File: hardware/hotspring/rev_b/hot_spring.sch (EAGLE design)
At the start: 27 parts, among them J1 GECKO_POWER_SUPPLY_CONN, J2 JUMPER-31-2, Q1 MOSFET-NCHANNELSMD, Q2 MOSFET-NCHANNELSMD, Q3 DUAL_MOSFET_NP, T1 LPR6235-752SMR, T2 LPR6235-752SMR, U1 LTC3109EUF

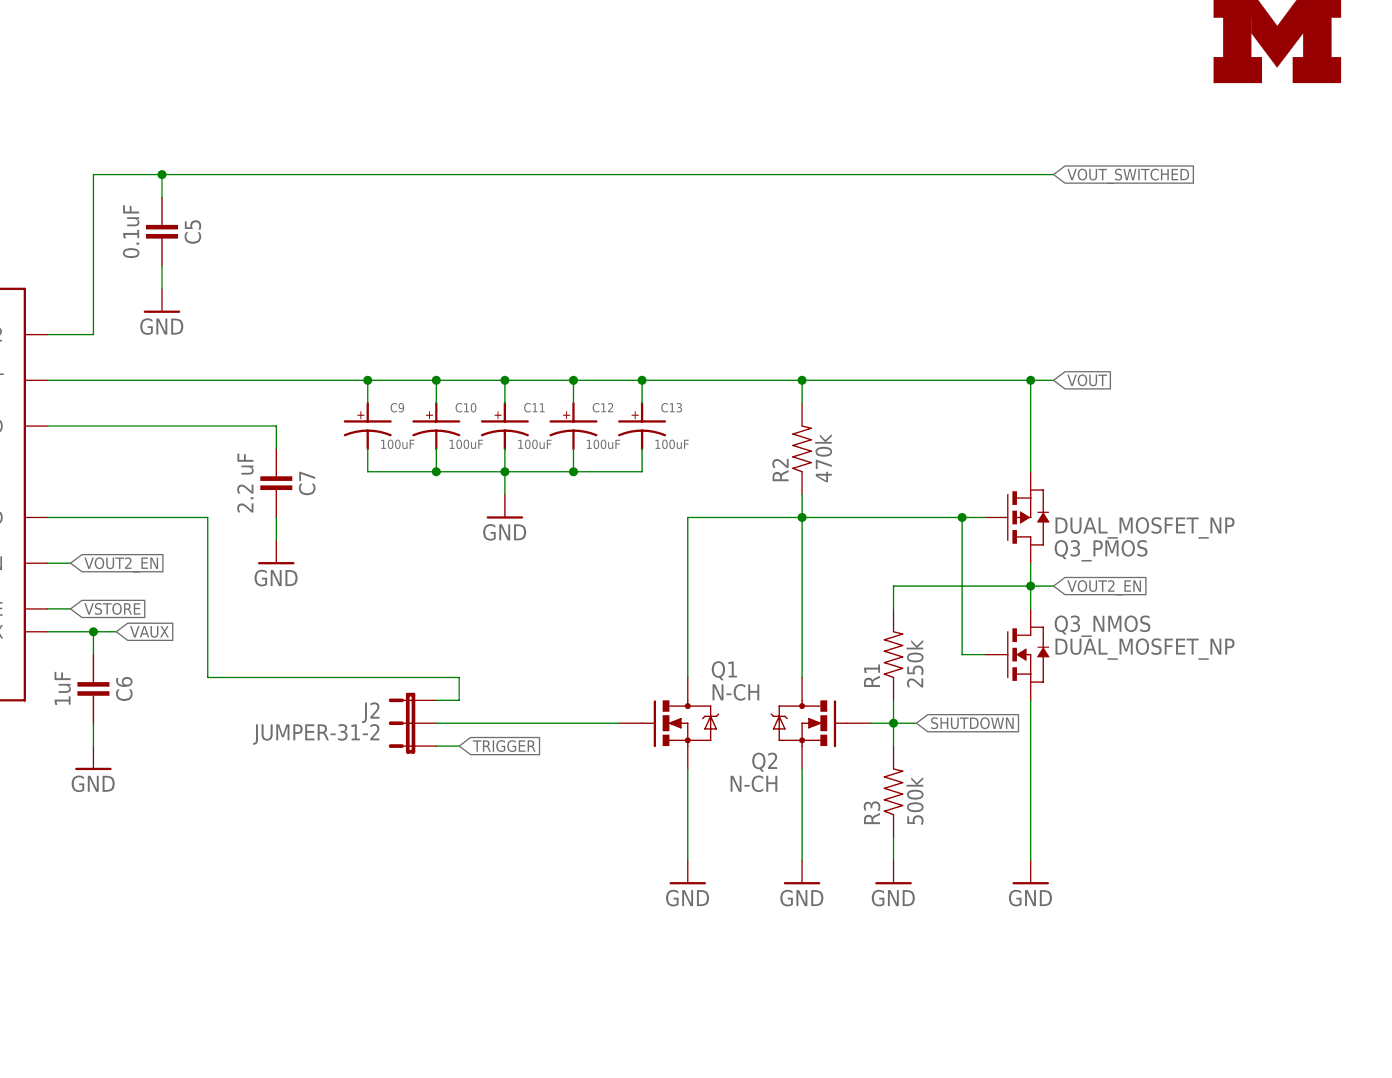
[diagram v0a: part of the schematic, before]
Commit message: hot spring updates
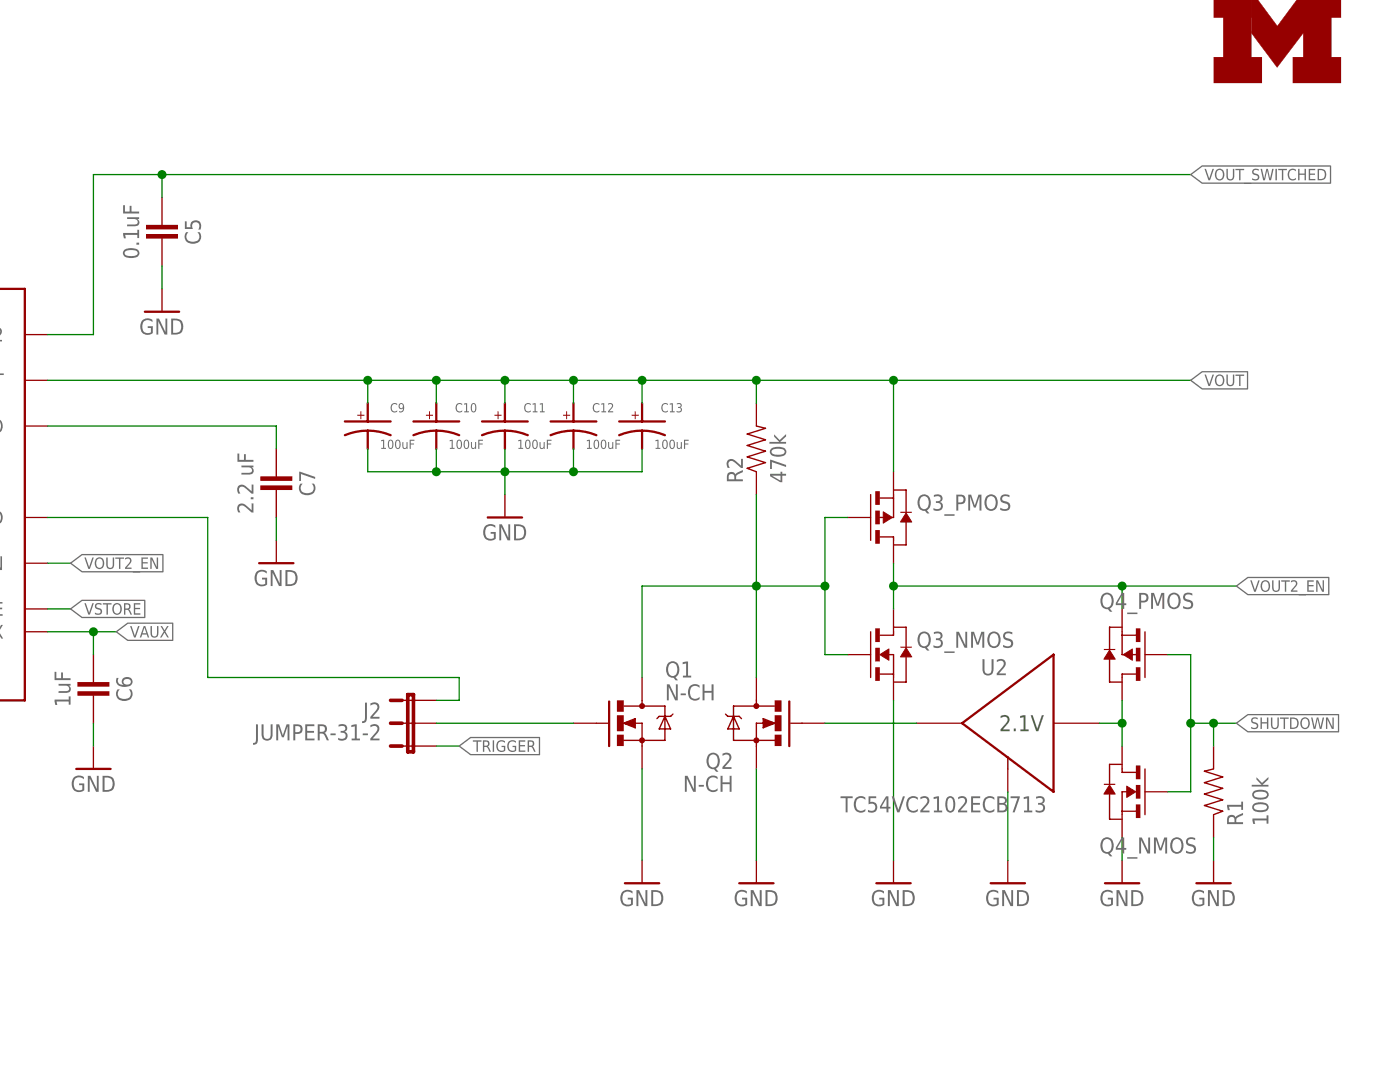
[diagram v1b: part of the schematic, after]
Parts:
- removed R3: 500k, passives:RESISTOR0402_RES
- added Q4: DUAL_MOSFET_NP, fets:DUAL_MOSFET_NP
- added U2: TC54VC2102ECB713, chips:TC54VC2102ECB713
- R1: value 250k -> 100k; DIGIKEY RHM249KCDCT-ND -> RHM100KCDCT-ND
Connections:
- new net N$13: Q2.G, U2.OUT
- new net N$5: Q4_NMOS.D, Q4_PMOS.D, U2.IN
- net GND: now also Q4_NMOS.S, R1.1, U2.GND; no longer R3.1
- net SHUTDOWN: now also Q4_NMOS.G, Q4_PMOS.G, R1.2; no longer Q2.G, R1.1, R3.2
- net VOUT2_EN: now also Q4_PMOS.S; no longer R1.2
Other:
- note added: "2.1V"
- moved on the sheet: Q1, Q2, Q3_NMOS, Q3_PMOS, R1, R2
